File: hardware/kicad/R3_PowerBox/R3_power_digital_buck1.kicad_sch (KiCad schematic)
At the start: 10 parts, among them U1 TPS62132RGTR

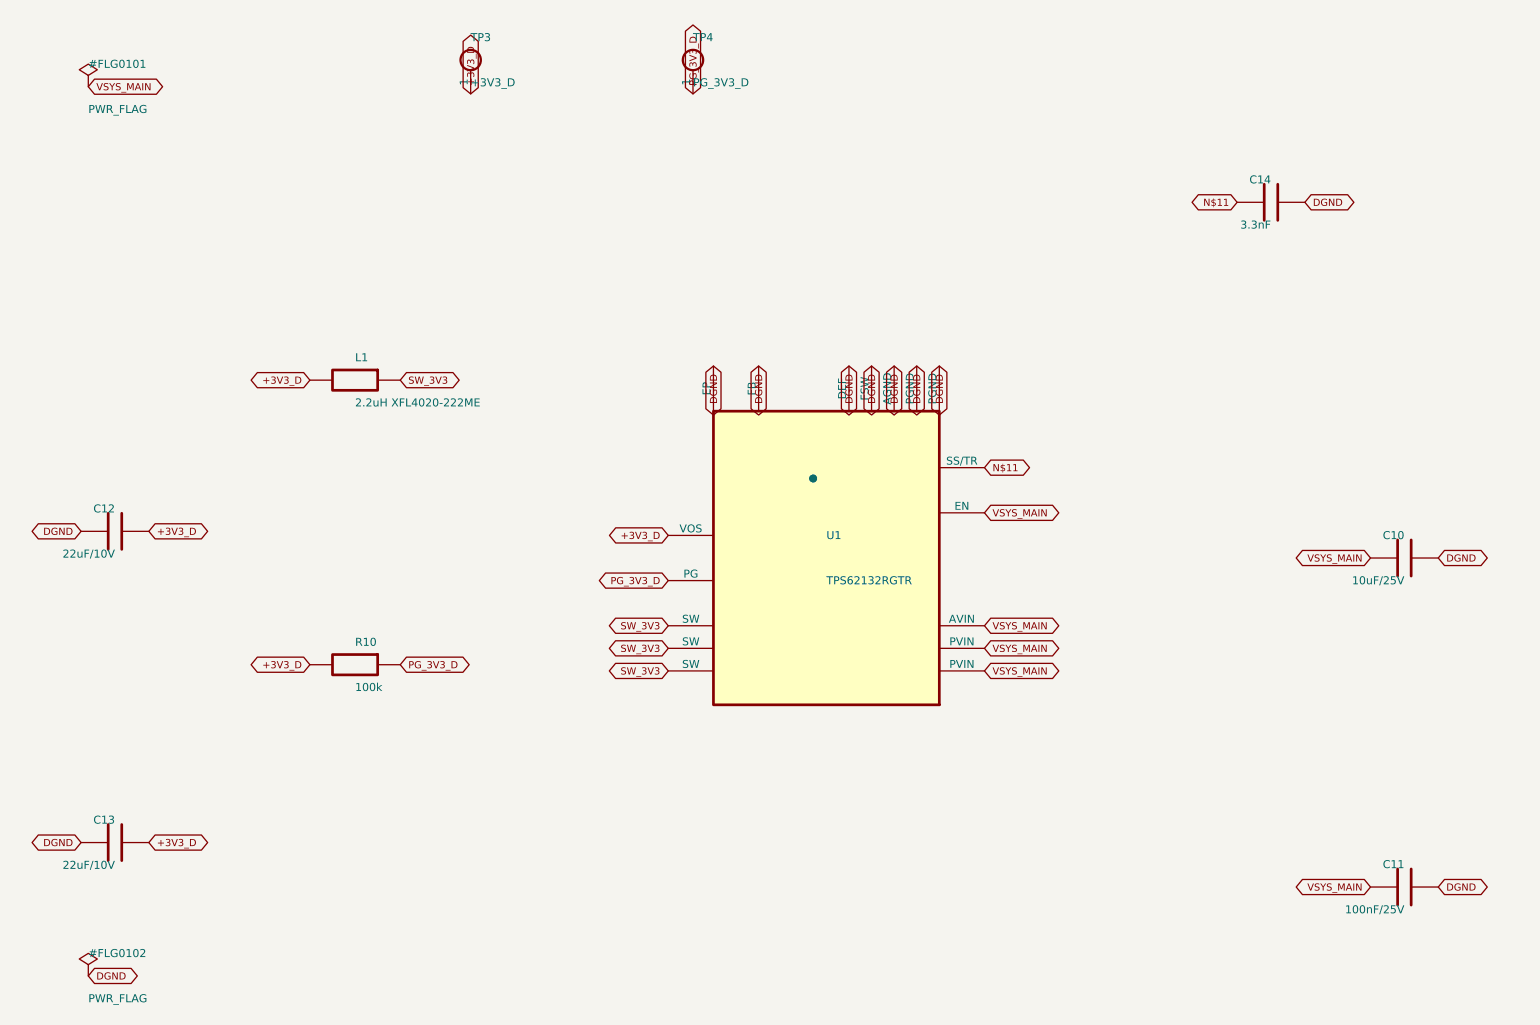
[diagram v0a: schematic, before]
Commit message: Rev.A review fixes: local charger power-stage reroute checkpoint
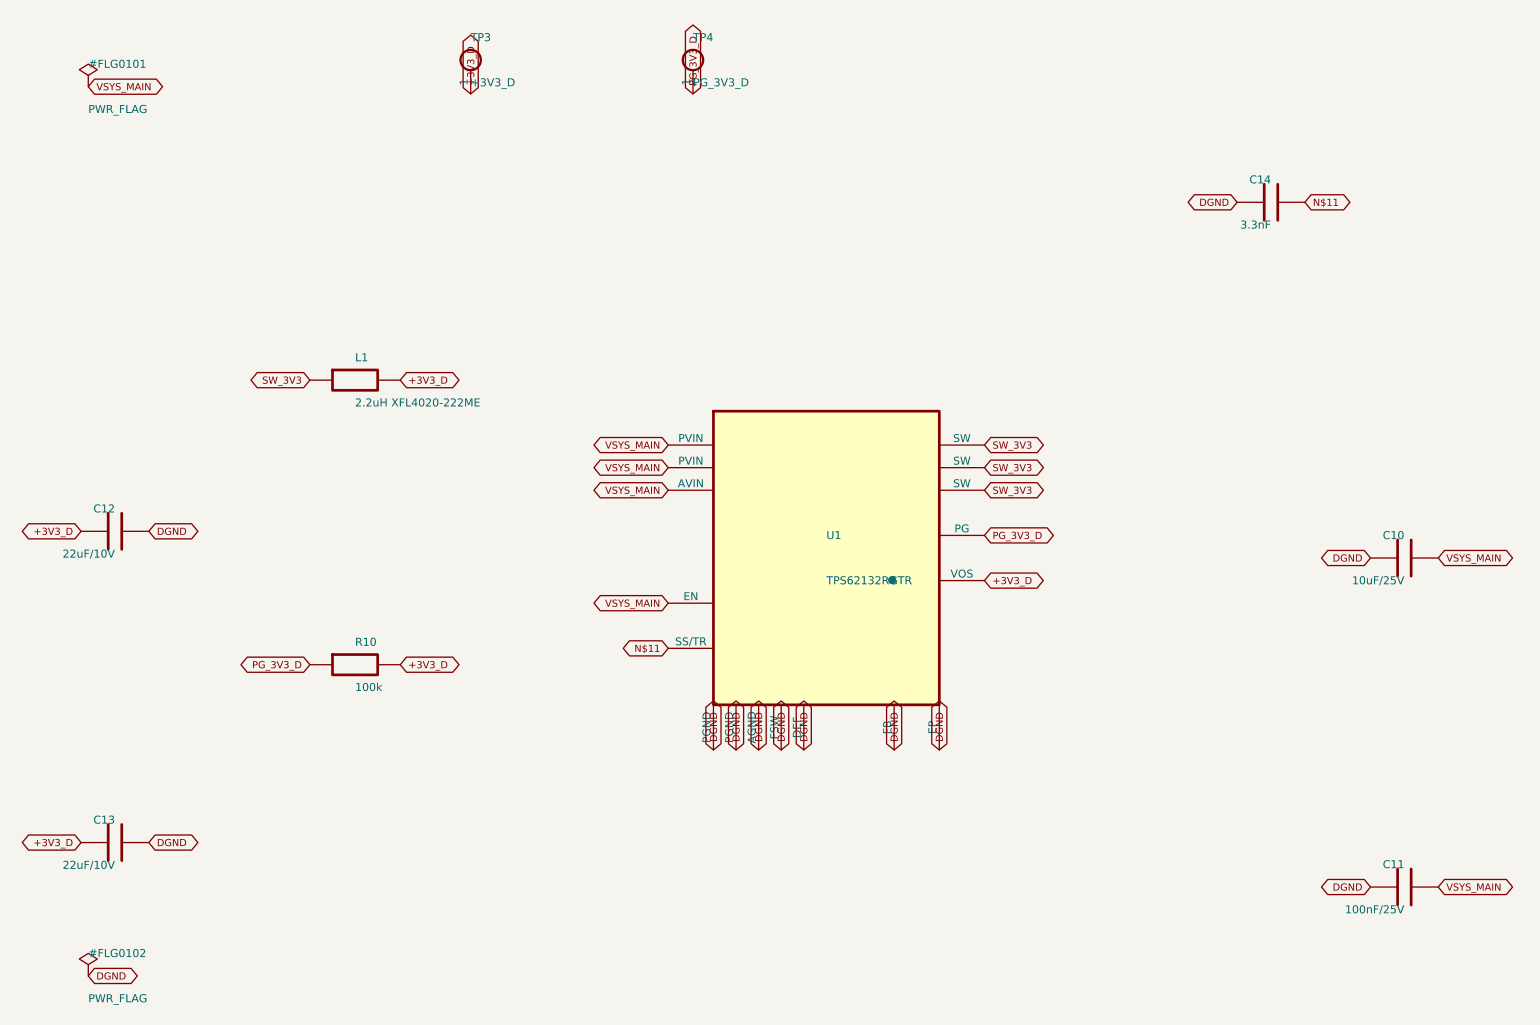
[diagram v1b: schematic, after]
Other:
- moved on the sheet: C10, C11, C12, C13, C14, L1, R10, U1
